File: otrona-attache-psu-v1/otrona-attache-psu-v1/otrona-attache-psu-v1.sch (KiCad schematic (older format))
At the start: 17 parts, among them J1 VIDEO, J2 CPU, J3 DRIVES, J4 15V_CONV, J5 ATX-24, J6 PWR, J7 FAN

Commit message: [otrona] Update schematic, layout, part selection
so far so good... now to print it out and see
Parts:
- C1, C2, C3, C4: footprint (none) -> Capacitor_THT:CP_Radial_D10.0mm_P5.00mm
- J1: footprint (none) -> Connector_Phoenix_MSTB:PhoenixContact_MSTBVA_2,5_5-G-5,08_1x05_P5.08mm_Vertical
- J2: footprint (none) -> Connector_Phoenix_MSTB:PhoenixContact_MSTBVA_2,5_12-G-5,08_1x12_P5.08mm_Vertical
- J3: footprint (none) -> Connector_Phoenix_MSTB:PhoenixContact_MSTBVA_2,5_8-G-5,08_1x08_P5.08mm_Vertical
- J4: footprint (none) -> Connector_PinHeader_2.54mm:PinHeader_1x04_P2.54mm_Horizontal
- J5: footprint (none) -> Connector_Molex:Molex_Mini-Fit_Jr_5566-24A2_2x12_P4.20mm_Vertical
- J6, J7: footprint (none) -> Connector_PinHeader_2.54mm:PinHeader_1x02_P2.54mm_Horizontal
- L1, L2, L3, L4, L5, L6: footprint (none) -> Inductor_THT:L_Axial_L11.0mm_D4.5mm_P15.24mm_Horizontal_Fastron_MECC

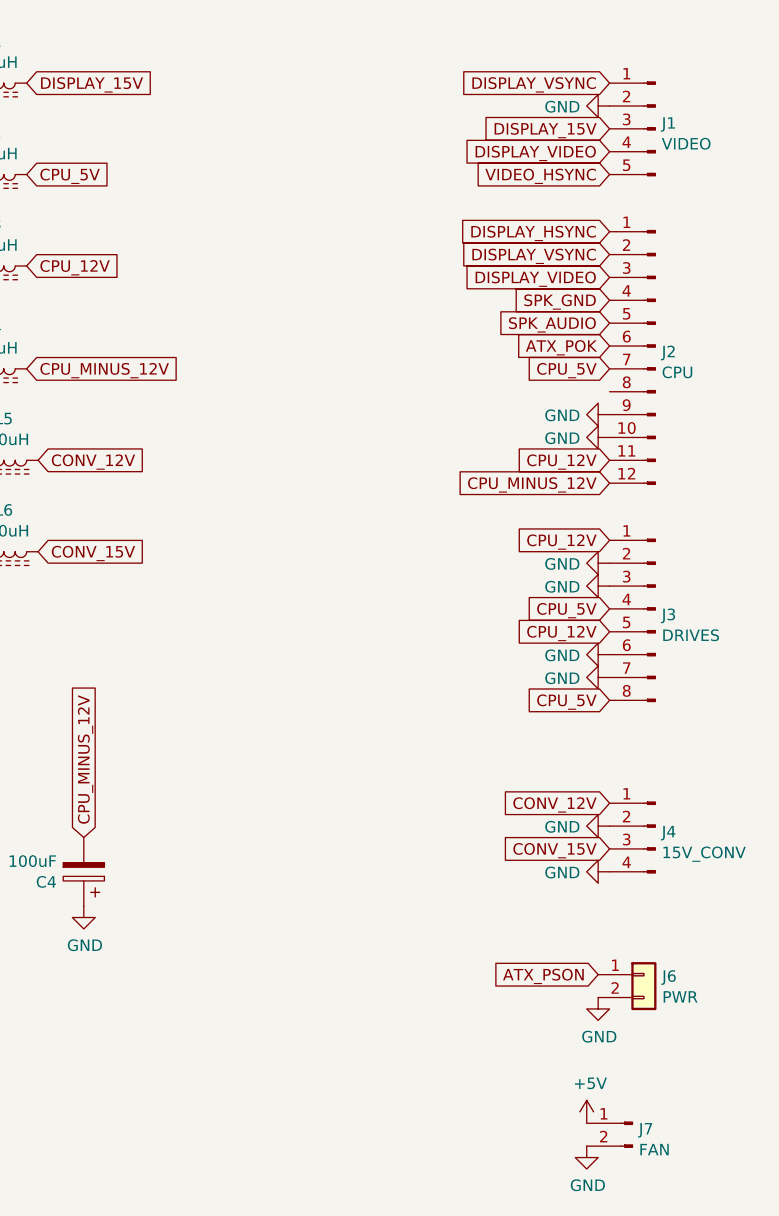
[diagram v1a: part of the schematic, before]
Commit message: [otrona] ok fine i routed the damned board
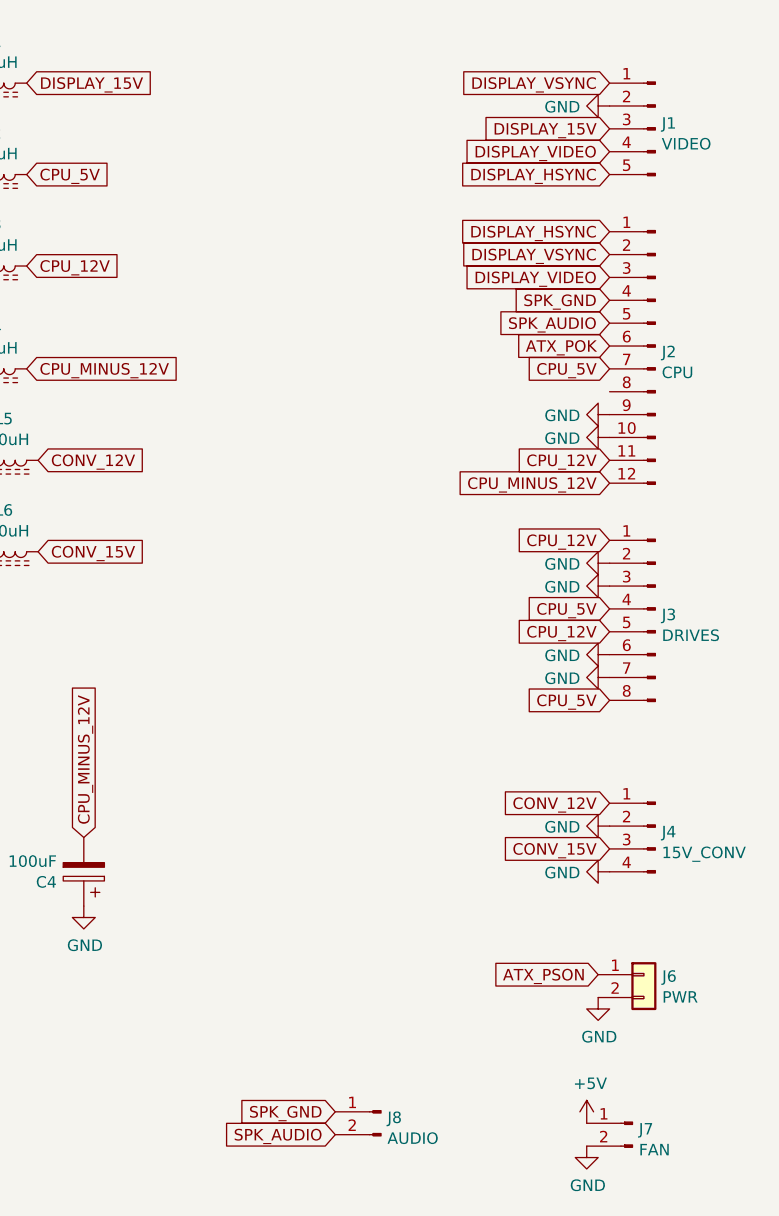
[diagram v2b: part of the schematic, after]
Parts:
- added J8: AUDIO, Connector_PinHeader_2.54mm:PinHeader_1x02_P2.54mm_Horizontal, symbol Connector:Conn_01x02_Male
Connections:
- net VIDEO_HSYNC is gone; now on net DISPLAY_HSYNC: J1.5 (Pin_5)
- net SPK_AUDIO: now also J8.2 (Pin_2)
- net SPK_GND: now also J8.1 (Pin_1)
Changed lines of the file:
@@
 DISPLAY_VIDEO
 Text GLabel 9800 1600 0    50   Input ~ 0
-VIDEO_HSYNC
+DISPLAY_HSYNC
 $Comp
 L power:GND #PWR0104
@@
 	1    0    0    -1
 $EndComp
+$Comp
+L Connector:Conn_01x02_Male J8
+U 1 1 62824E1A
+P 8800 5700
+F 0 "J8" H 8772 5674 50  0000 R CNN
+F 1 "AUDIO" H 8772 5583 50  0000 R CNN
+F 2 "Connector_PinHeader_2.54mm:PinHeader_1x02_P2.54mm_Horizontal" H 8800 5700 50  0001 C CNN
+F 3 "~" H 8800 5700 50  0001 C CNN
+	1    8800 5700
+	-1   0    0    -1
+$EndComp
+Text GLabel 8600 5800 0    50   Input ~ 0
+SPK_AUDIO
+Text GLabel 8600 5700 0    50   Input ~ 0
+SPK_GND
 $EndSCHEMATC
